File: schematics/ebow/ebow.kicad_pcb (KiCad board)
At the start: 2 copper layers, 70 x 30 mm, 18 parts, among them SW1 SW_SPDT, U1 LM386

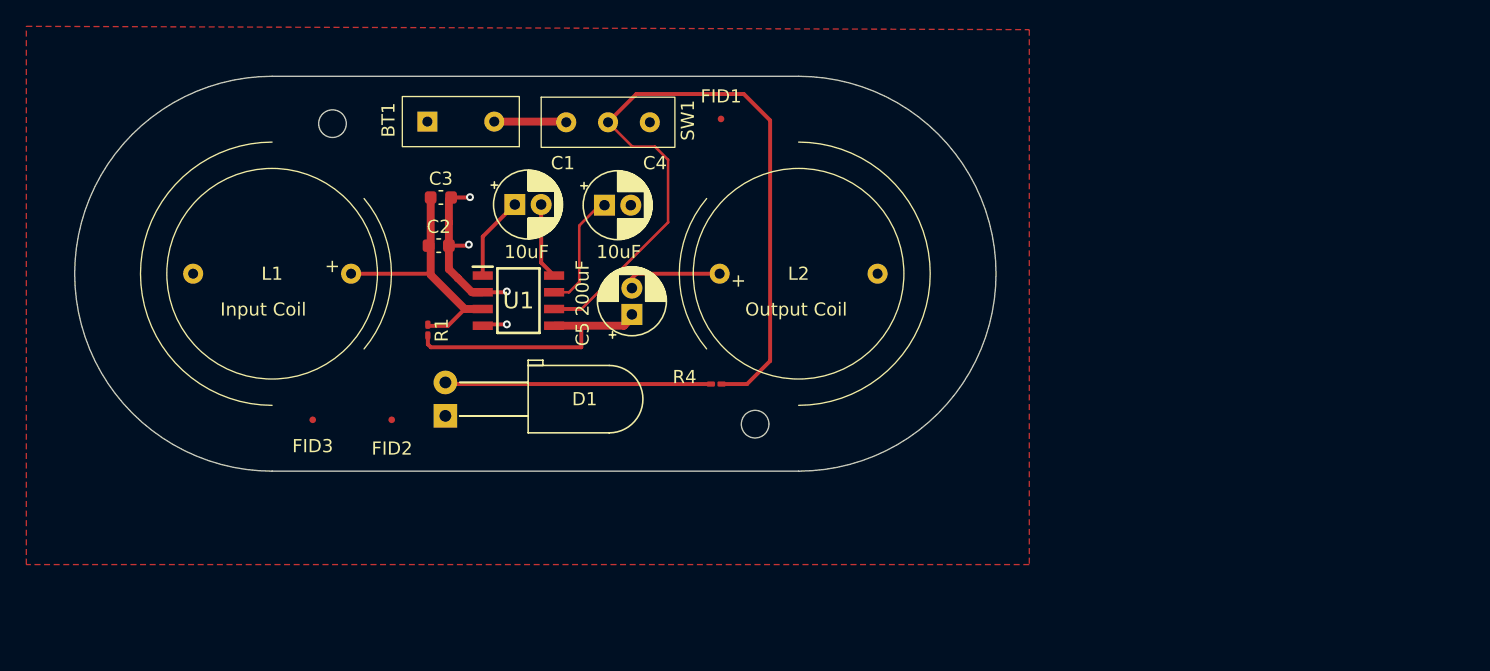
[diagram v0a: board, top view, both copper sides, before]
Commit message: added board characteristics
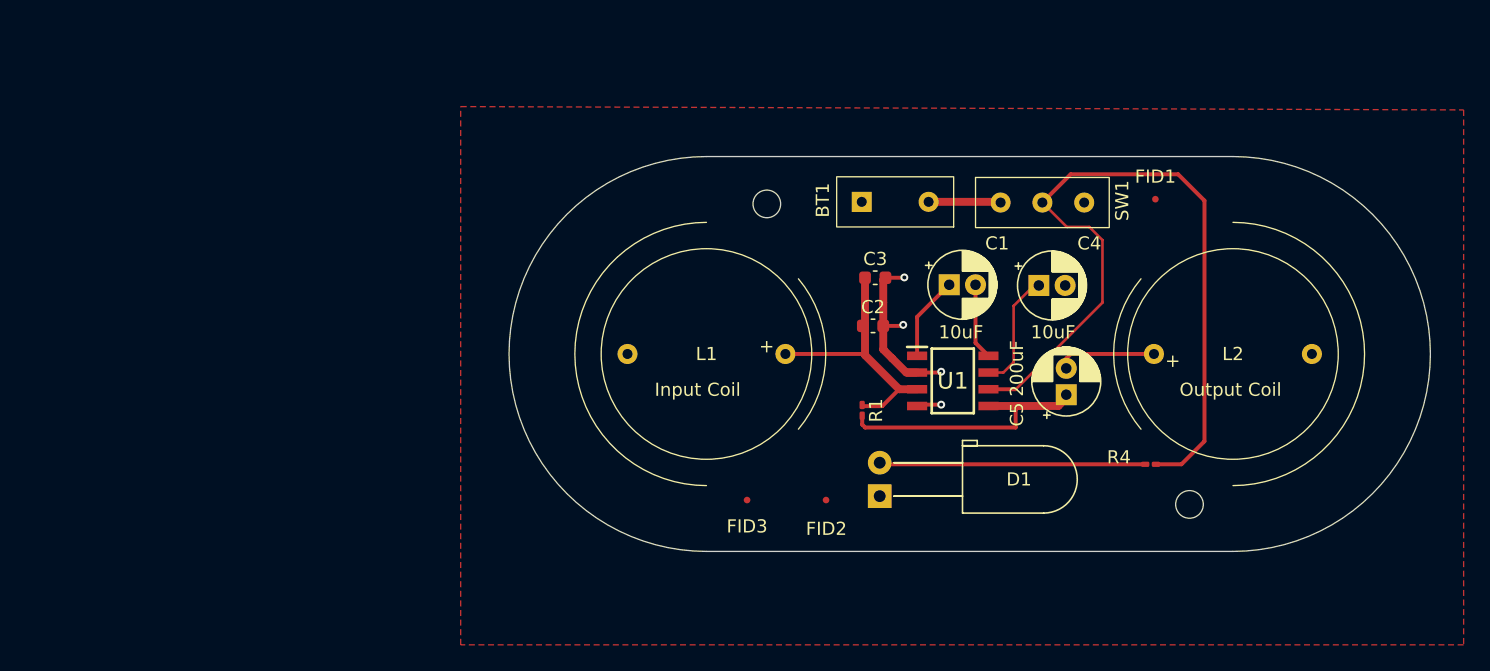
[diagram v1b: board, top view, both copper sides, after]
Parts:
- moved BT1 33.6 mm to (208.2, 99.3)
- moved C1 33.6 mm to (212.4, 105.7)
- moved C2 33.6 mm to (206.6, 108.9)
- moved C3 33.6 mm to (206.7, 105.2)
- moved C4 33.6 mm to (219.2, 105.8)
- moved C5 33.6 mm to (221.2, 114.1)
- moved D1 33.6 mm to (207.1, 121.8)
- moved FID1 33.6 mm to (228.0, 99.2)
- moved FID2 33.6 mm to (203.0, 122.1)
- moved FID3 33.6 mm to (197.0, 122.1)
- moved H1 33.6 mm to (230.6, 122.4)
- moved H2 33.6 mm to (198.5, 99.6)
- moved L1 33.6 mm to (193.9, 111.0)
- moved L2 33.6 mm to (233.9, 111.0)
- moved R1 33.6 mm to (205.7, 115.3)
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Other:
- board text added: "0"
- board text added: "0 mm"
- board text added: "0.0000 mm / 0.0000 mm"
- board text added: "0.01 mm"
- board text added: "0.02"
- board text added: "0.035 mm"
- board text added: "0.3000 mm"
- board text added: "1"
- board text added: "1.51 mm"
- board text added: "1.6000 mm"
- board text added: "2"
- board text added: "3.3"
- board text added: "4.5"
- board text added: "70.0050 mm x 30.0000 mm"
- board text added: "B.Cu"
- board text added: "B.Mask"
- board text added: "B.Paste"
- board text added: "B.Silkscreen"
- board text added: "BOARD CHARACTERISTICS"
- board text added: "Board Thickness:"
- board text added: "Board overall dimensions:"
- board text added: "Bottom Silk Screen"
- board text added: "Bottom Solder Mask"
- board text added: "Bottom Solder Paste"
- board text added: "Castellated pads:"
- board text added: "Color"
- board text added: "Copper Finish:"
- board text added: "Copper Layer Count:"
- board text added: "Dielectric"
- board text added: "Edge card connectors:"
- board text added: "Epsilon R"
- board text added: "F.Cu"
- board text added: "F.Mask"
- board text added: "F.Paste"
- board text added: "F.Silkscreen"
- board text added: "FR4"
- board text added: "Impedance Control:"
- board text added: "Layer Name"
- board text added: "Loss Tangent"
- board text added: "Material"
- board text added: "Min hole diameter:"
- board text added: "Min track/spacing:"
- board text added: "No"
- board text added: "None"
- board text added: "Not specified"
- board text added: "Plated Board Edge:"
- board text added: "Thickness (mm)"
- board text added: "Top Silk Screen"
- board text added: "Top Solder Mask"
- board text added: "Top Solder Paste"
- board text added: "Type"
- board text added: "copper"
- board text added: "core"
